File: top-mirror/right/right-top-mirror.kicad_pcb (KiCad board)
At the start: 2 copper layers, 171 x 95 mm, 39 parts

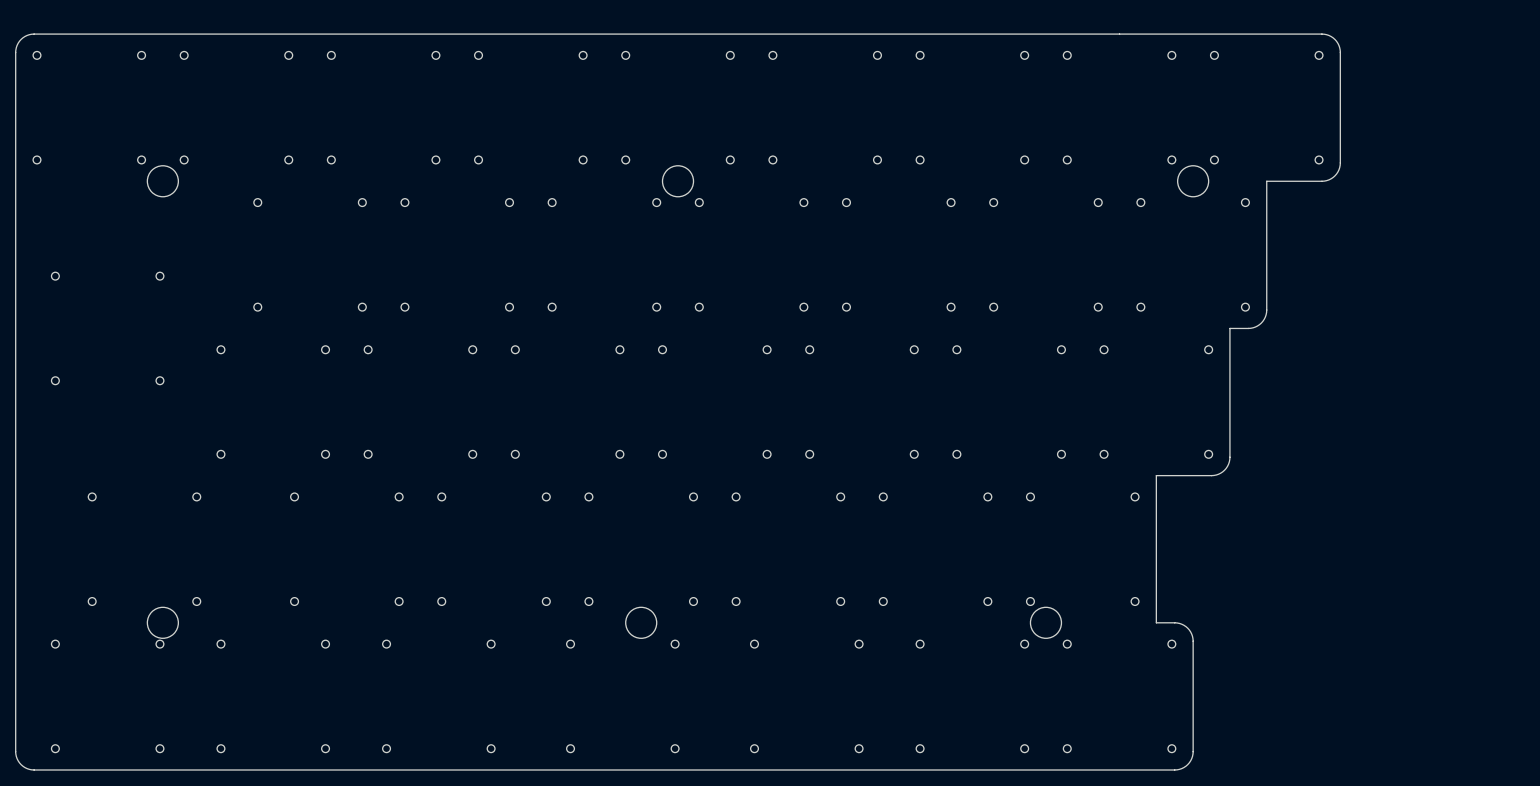
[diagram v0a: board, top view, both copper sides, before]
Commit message: rev1 release
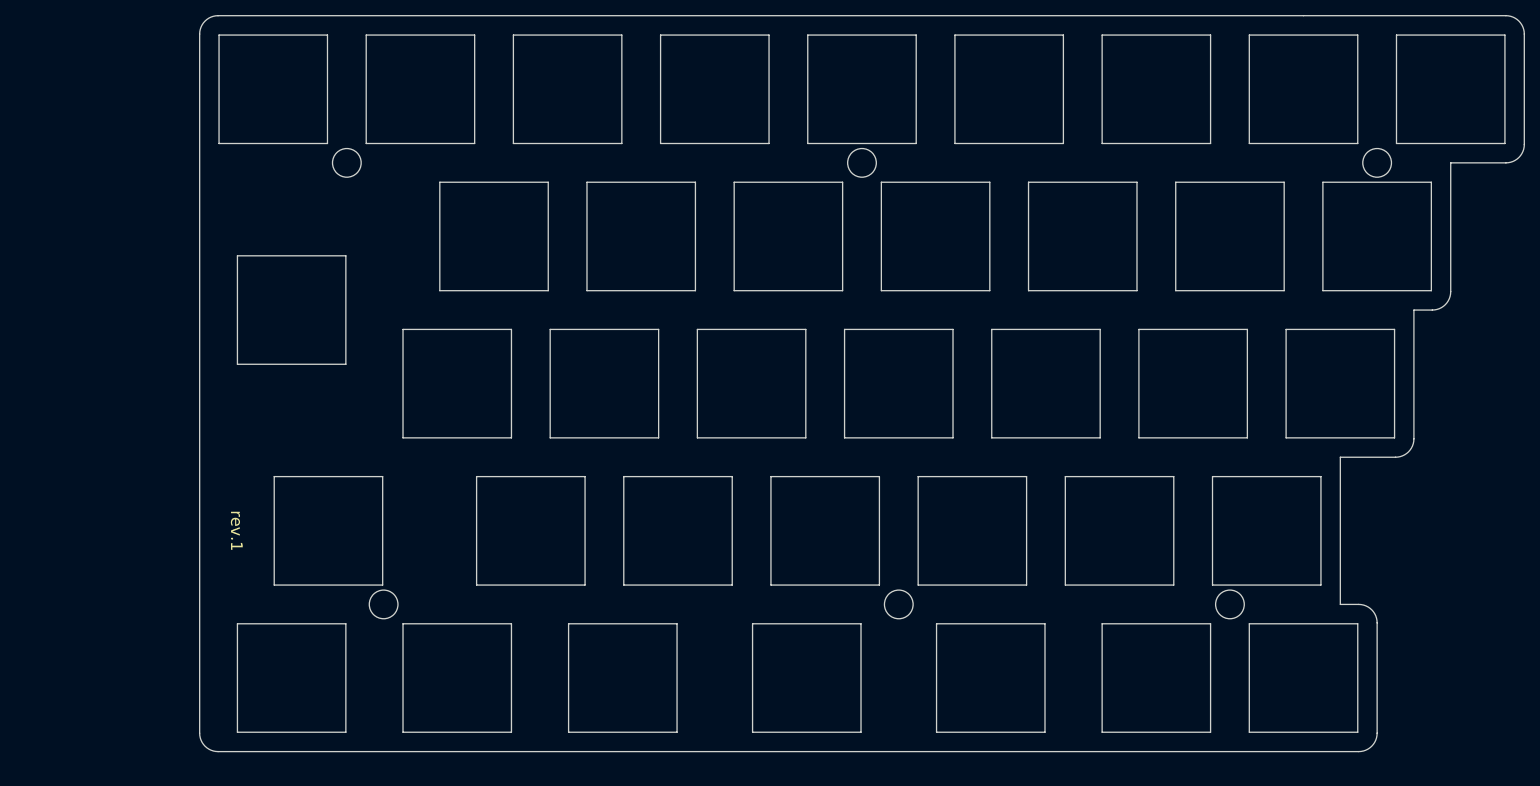
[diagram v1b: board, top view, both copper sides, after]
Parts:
- removed the MX_CUTOUT at (180.5, 130.6)
- removed the MX_CUTOUT at (85.5, 54.6)
- removed the MX_CUTOUT at (104.5, 54.6)
- removed the MX_CUTOUT at (123.5, 54.6)
- removed the MX_CUTOUT at (142.5, 54.6)
- removed the MX_CUTOUT at (161.5, 54.6)
- removed the MX_CUTOUT at (180.5, 54.6)
- removed the MX_CUTOUT at (199.5, 54.6)
- removed the MX_CUTOUT at (190.0, 73.6)
- removed the MX_CUTOUT at (171.0, 73.6)
- removed the MX_CUTOUT at (152.0, 73.6)
- removed the MX_CUTOUT at (161.5, 130.6)
- removed the MX_CUTOUT at (133.0, 73.6)
- removed the MX_CUTOUT at (114.0, 73.6)
- removed the MX_CUTOUT at (95.0, 73.6)
- removed the MX_CUTOUT at (76.0, 73.6)
- removed the MX_CUTOUT at (71.2, 92.6)
- removed the MX_CUTOUT at (90.2, 92.6)
- removed the MX_CUTOUT at (109.2, 92.6)
- removed the MX_CUTOUT at (128.2, 92.6)
- removed the MX_CUTOUT at (147.2, 92.6)
- removed the MX_CUTOUT at (166.2, 92.6)
- removed the MX_CUTOUT at (140.1, 130.6)
- removed the MX_CUTOUT at (185.2, 92.6)
- removed the MX_CUTOUT at (175.8, 111.6)
- removed the MX_CUTOUT at (156.8, 111.6)
- removed the MX_CUTOUT at (137.8, 111.6)
- removed the MX_CUTOUT at (118.8, 111.6)
- removed the MX_CUTOUT at (99.8, 111.6)
- removed the MX_CUTOUT at (80.8, 111.6)
- removed the MX_CUTOUT at (54.6, 111.6)
- removed the MX_CUTOUT at (49.9, 83.1)
- removed the MX_CUTOUT at (116.4, 130.6)
- removed the MX_CUTOUT at (92.6, 130.6)
- removed the MX_CUTOUT at (71.2, 130.6)
- removed the MX_CUTOUT at (49.9, 130.6)
- removed the MX_CUTOUT at (47.5, 54.6)
- removed the MX_CUTOUT at (66.5, 54.6)
- added MX_CUTOUT: VAL**, lib:MX_CUTOUT, B.Cu at (180.5, 109.2)
- added MX_CUTOUT: VAL**, lib:MX_CUTOUT, B.Cu at (223.2, 52.2)
- added MX_CUTOUT: VAL**, lib:MX_CUTOUT, B.Cu at (99.8, 71.2)
- added MX_CUTOUT: VAL**, lib:MX_CUTOUT, B.Cu at (199.5, 109.2)
- added MX_CUTOUT: VAL**, lib:MX_CUTOUT, B.Cu at (78.4, 109.2)
- added MX_CUTOUT: VAL**, lib:MX_CUTOUT, B.Cu at (204.2, 52.2)
- added MX_CUTOUT: VAL**, lib:MX_CUTOUT, B.Cu at (73.6, 80.8)
- added MX_CUTOUT: VAL**, lib:MX_CUTOUT, B.Cu at (213.8, 71.2)
- added MX_CUTOUT: VAL**, lib:MX_CUTOUT, B.Cu at (161.5, 109.2)
- added MX_CUTOUT: VAL**, lib:MX_CUTOUT, B.Cu at (133.0, 90.2)
- added MX_CUTOUT: VAL**, lib:MX_CUTOUT, B.Cu at (194.8, 71.2)
- added MX_CUTOUT: VAL**, lib:MX_CUTOUT, B.Cu at (118.8, 71.2)
- added MX_CUTOUT: VAL**, lib:MX_CUTOUT, B.Cu at (171.0, 90.2)
- added MX_CUTOUT: VAL**, lib:MX_CUTOUT, B.Cu at (209.0, 90.2)
- added MX_CUTOUT: VAL**, lib:MX_CUTOUT, B.Cu at (190.0, 90.2)
- added MX_CUTOUT: VAL**, lib:MX_CUTOUT, B.Cu at (156.8, 71.2)
- added MX_CUTOUT: VAL**, lib:MX_CUTOUT, B.Cu at (152.0, 90.2)
- added MX_CUTOUT: VAL**, lib:MX_CUTOUT, B.Cu at (95.0, 128.2)
- added MX_CUTOUT: VAL**, lib:MX_CUTOUT, B.Cu at (73.6, 128.2)
- added MX_CUTOUT: VAL**, lib:MX_CUTOUT, B.Cu at (71.2, 52.2)
- added MX_CUTOUT: VAL**, lib:MX_CUTOUT, B.Cu at (90.2, 52.2)
- added MX_CUTOUT: VAL**, lib:MX_CUTOUT, B.Cu at (109.2, 52.2)
- added MX_CUTOUT: VAL**, lib:MX_CUTOUT, B.Cu at (175.8, 71.2)
- added MX_CUTOUT: VAL**, lib:MX_CUTOUT, B.Cu at (128.2, 52.2)
- added MX_CUTOUT: VAL**, lib:MX_CUTOUT, B.Cu at (104.5, 109.2)
- added MX_CUTOUT: VAL**, lib:MX_CUTOUT, B.Cu at (147.2, 52.2)
- added MX_CUTOUT: VAL**, lib:MX_CUTOUT, B.Cu at (142.5, 109.2)
- added MX_CUTOUT: VAL**, lib:MX_CUTOUT, B.Cu at (204.2, 128.2)
- added MX_CUTOUT: VAL**, lib:MX_CUTOUT, B.Cu at (140.1, 128.2)
- added MX_CUTOUT: VAL**, lib:MX_CUTOUT, B.Cu at (185.2, 128.2)
- added MX_CUTOUT: VAL**, lib:MX_CUTOUT, B.Cu at (116.4, 128.2)
- added MX_CUTOUT: VAL**, lib:MX_CUTOUT, B.Cu at (163.9, 128.2)
- added MX_CUTOUT: VAL**, lib:MX_CUTOUT, B.Cu at (185.2, 52.2)
- added MX_CUTOUT: VAL**, lib:MX_CUTOUT, B.Cu at (166.2, 52.2)
- added MX_CUTOUT: VAL**, lib:MX_CUTOUT, B.Cu at (114.0, 90.2)
- added MX_CUTOUT: VAL**, lib:MX_CUTOUT, B.Cu at (137.8, 71.2)
- added MX_CUTOUT: VAL**, lib:MX_CUTOUT, B.Cu at (95.0, 90.2)
- added MX_CUTOUT: VAL**, lib:MX_CUTOUT, B.Cu at (123.5, 109.2)
- added REF**: MountingHole_3.7mm, MountingHole:MountingHole_3.7mm, B.Cu at (147.2, 61.8)
- added REF**: MountingHole_3.7mm, MountingHole:MountingHole_3.7mm, B.Cu at (152.0, 118.8)
- added REF**: MountingHole_3.7mm, MountingHole:MountingHole_3.7mm, B.Cu at (80.8, 61.8)
- added REF**: MountingHole_3.7mm, MountingHole:MountingHole_3.7mm, B.Cu at (85.5, 118.8)
- added REF**: MountingHole_3.7mm, MountingHole:MountingHole_3.7mm, B.Cu at (194.8, 118.8)
- added REF**: MountingHole_3.7mm, MountingHole:MountingHole_3.7mm, B.Cu at (213.8, 61.8)
- moved REF** 23.9 mm to (73.6, 80.8)
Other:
- outline, holes or cut-outs redrawn
- board text added: "rev.1"
